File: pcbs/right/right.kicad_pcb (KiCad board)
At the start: 2 copper layers, 135.8 x 108.4 mm, 70 parts

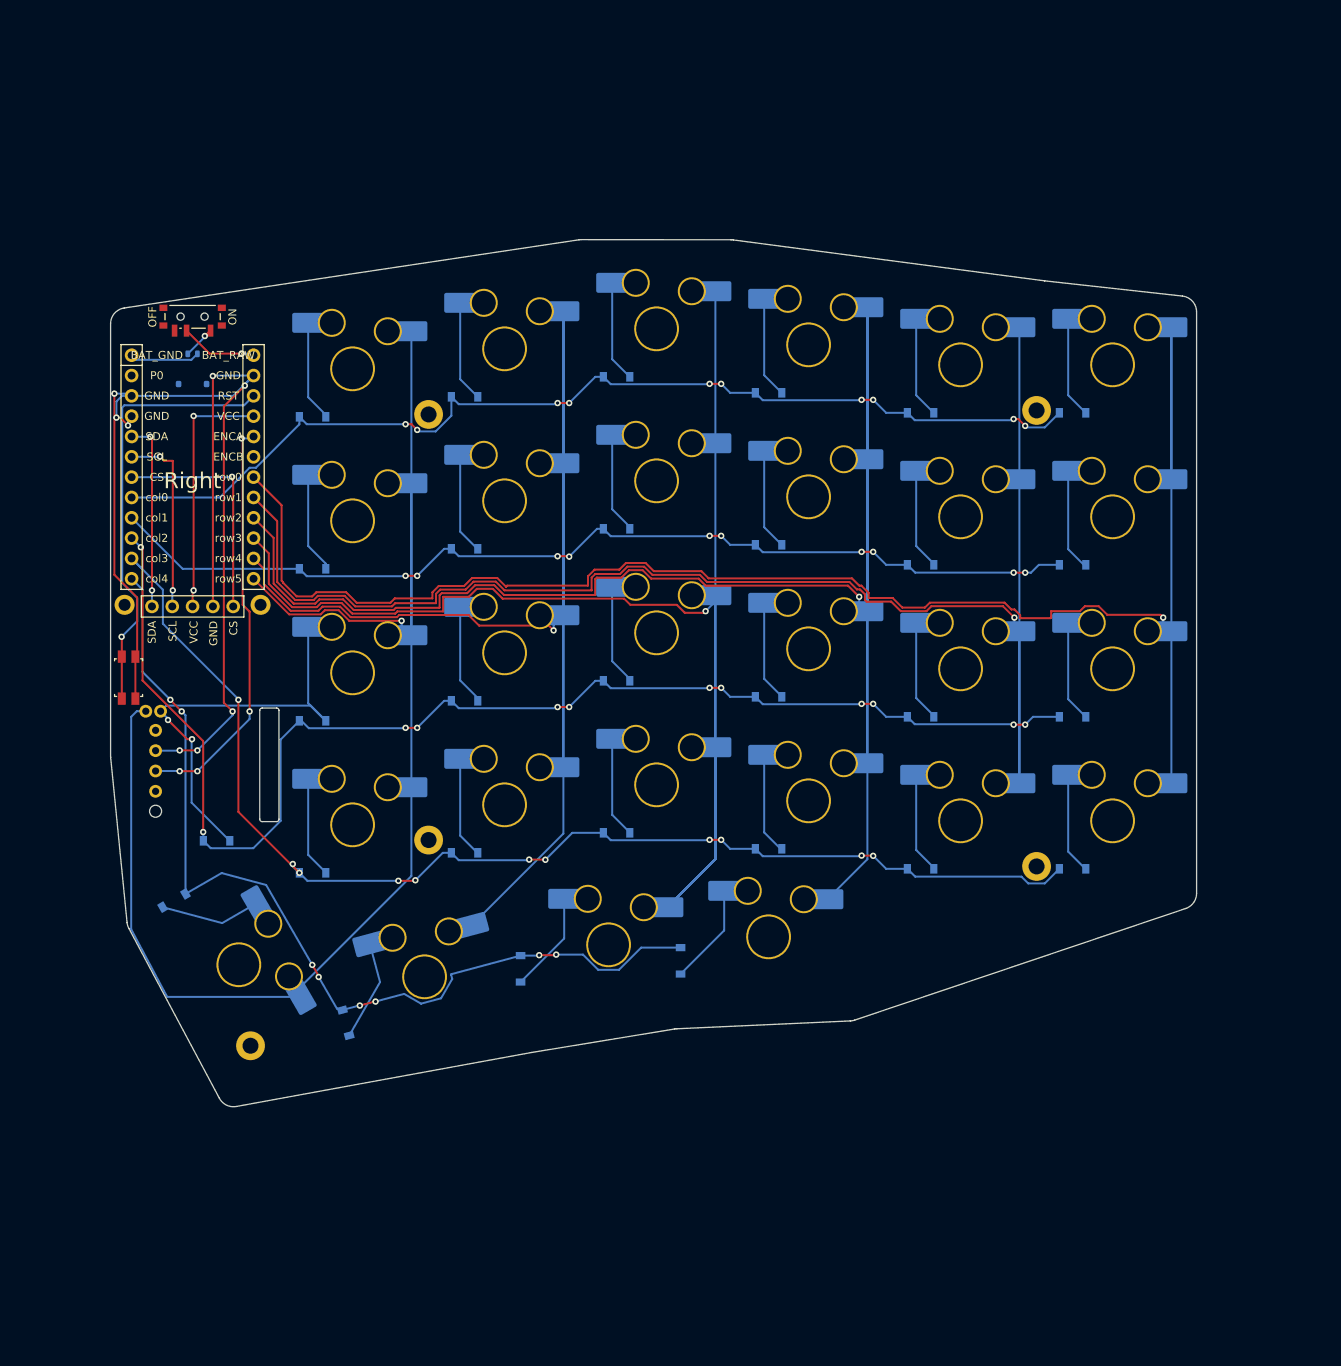
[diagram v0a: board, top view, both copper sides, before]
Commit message: added fill
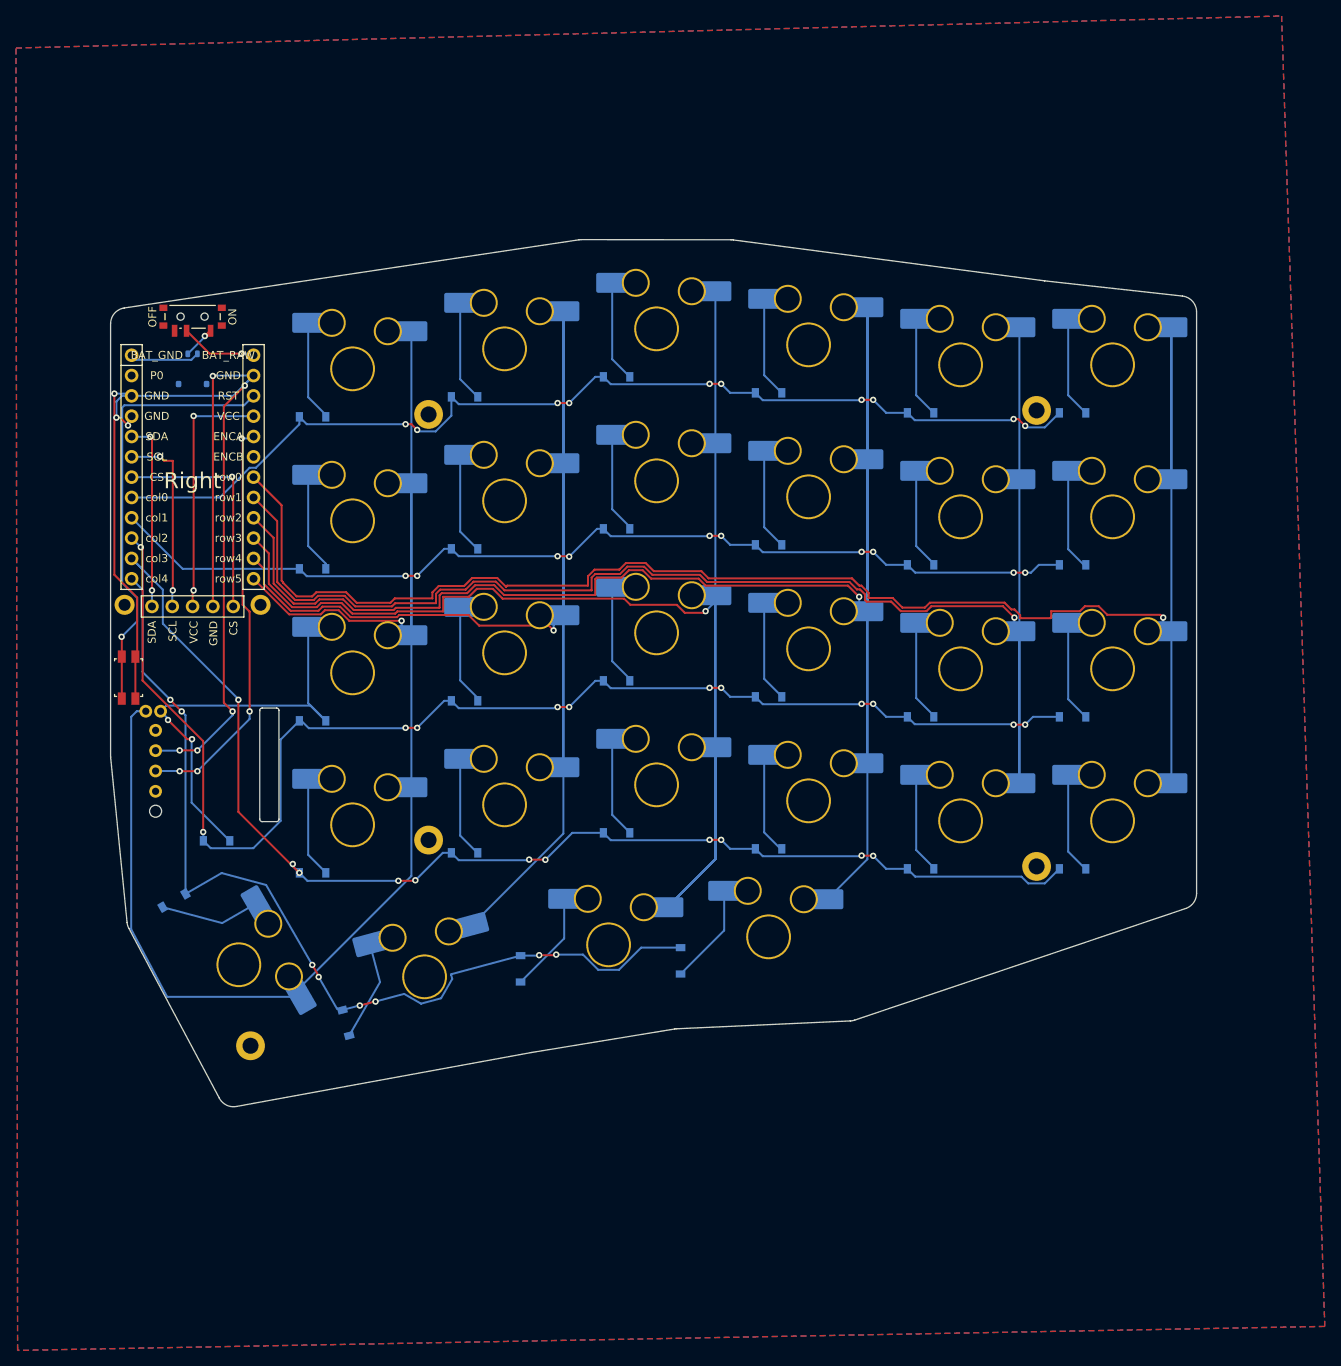
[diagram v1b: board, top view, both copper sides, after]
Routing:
- added copper zone on B.Cu, net (none)
- added copper zone on F.Cu, net (none)
